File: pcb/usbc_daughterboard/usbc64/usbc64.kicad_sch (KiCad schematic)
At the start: 5 parts, among them J1 USB_C_Receptacle_USB2.0

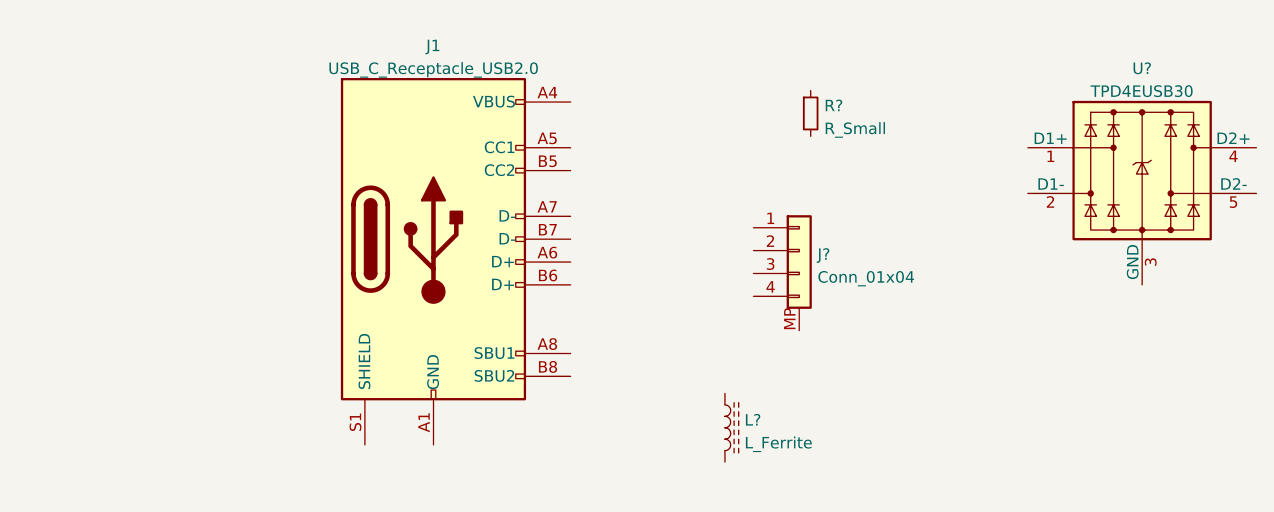
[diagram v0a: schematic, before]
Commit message: sch and pcb rough starts
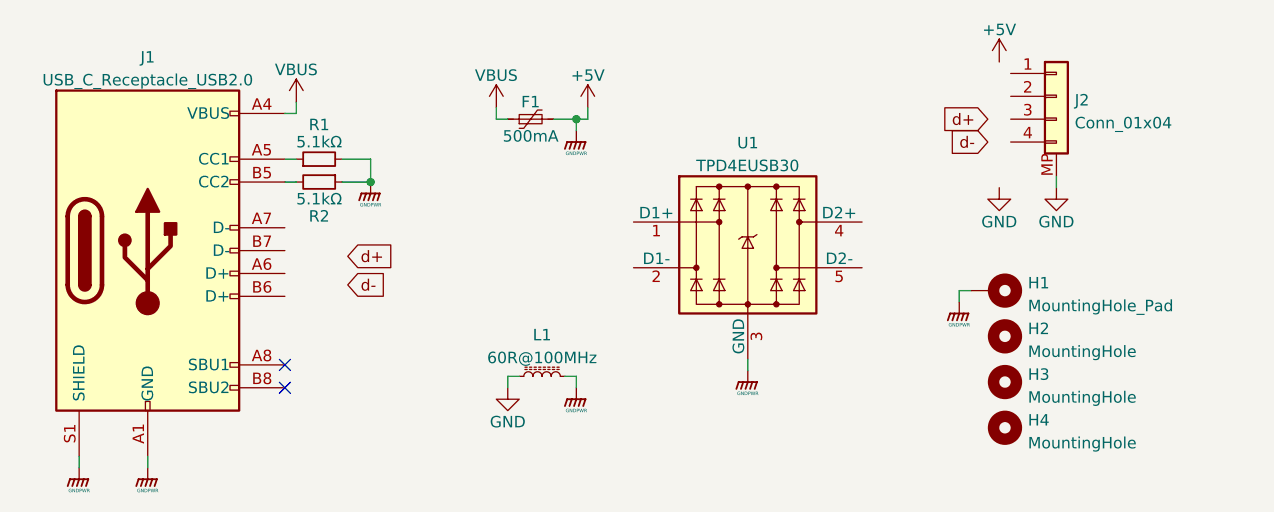
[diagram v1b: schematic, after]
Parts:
- removed R?: R_Small, symbol Device:R_Small
- added F1: 500mA, symbol Device:Polyfuse_Small
- added H1: MountingHole_Pad, symbol Mechanical:MountingHole_Pad
- added H2, H3, H4: MountingHole, symbol Mechanical:MountingHole
- added R1, R2: 5.1kΩ, Resistor_SMD:R_0805_2012Metric, symbol Device:R_Small
- J2: renamed from J?; footprint (none) -> Connector_JST:JST_SUR_SM04B-SURS-TF_1x04-1MP_P0.80mm_Horizontal
- L1: renamed from L?; value L_Ferrite -> 60R@100MHz; footprint (none) -> Inductor_SMD:L_1206_3216Metric; symbol Device:L_Ferrite -> Device:L_Ferrite_Small
- gave numbers to parts that had none: 1
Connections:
- net GND: now reaches L1.1
- net GND: now also J2.MP
- net +5V: now reaches L1.2
- net +5V: now also J1.A1 (GND), J1.A12 (GND), J1.B1 (GND), J1.B12 (GND), J1.S1 (SHIELD), U1.3 (GND), U1.8 (GND), F1.2, H1.1, R1.2, R2.1
- net VBUS: now reaches J1.A4 (VBUS), J1.A9 (VBUS), J1.B4 (VBUS), J1.B9 (VBUS)
- net VBUS: now also F1.1
- net at J1.A5 (CC1): now also R1.1
- net at J1.B5 (CC2): now also R2.2
- no-connect marks 0 -> 2
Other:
- moved on the sheet: J1, J2, U1
